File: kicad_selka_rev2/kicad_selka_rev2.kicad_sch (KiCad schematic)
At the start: 104 parts, among them J1 Conn_01x02_Pin, J10 Conn_01x01_Pin, J11 Conn_01x01_Pin, J12 Conn_01x01_Pin, J13 Conn_01x01_Pin, J14 Conn_01x01_Pin, J15 Conn_01x01_Pin, J16 Conn_01x01_Pin, J17 Conn_01x01_Pin, J18 Conn_01x01_Pin, J19 Conn_01x01_Pin, J2 Conn_01x01_Pin, J20 Conn_01x01_Pin, J3 Conn_01x01_Pin, J4 Conn_01x06_Pin, J5 Conn_01x01_Pin, J6 Conn_01x01_Pin, J7 Conn_01x01_Pin, J8 Conn_01x01_Pin, J9 Conn_01x01_Pin, Q1 NPN, U1 ATtiny861A-S

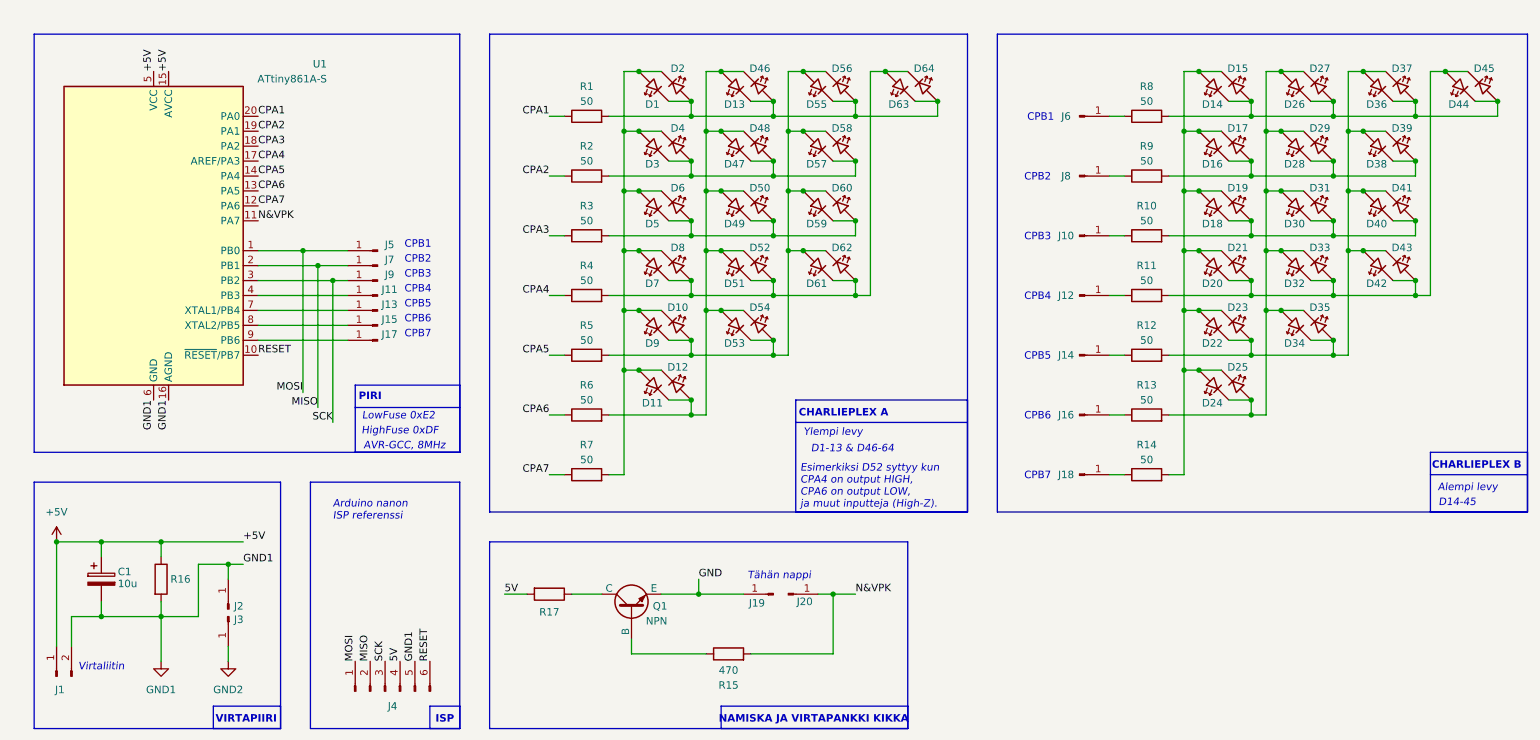
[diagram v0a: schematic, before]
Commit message: hiomista vaille rev
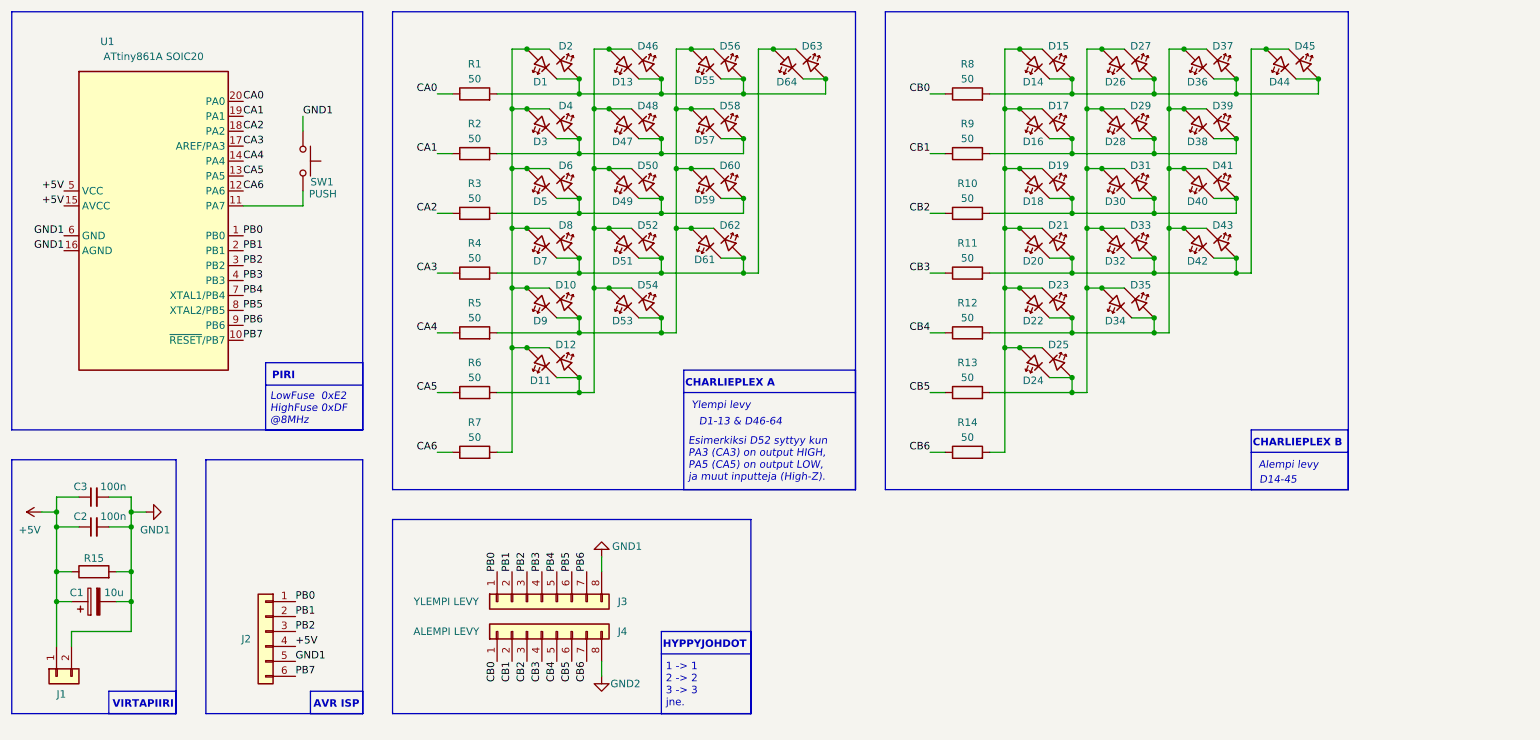
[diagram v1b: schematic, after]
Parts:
- removed J1: Conn_01x02_Pin, Connector_PinHeader_2.00mm:PinHeader_1x02_P2.00mm_Vertical, symbol Connector:Conn_01x02_Pin
- removed J10, J11, J12, J13, J14, J15, J16, J17, J18, J19, J2, J20, J3, J5, J6, J7, J8, J9: Conn_01x01_Pin, Connector_PinHeader_2.00mm:PinHeader_1x01_P2.00mm_Vertical, symbol Connector:Conn_01x01_Pin
- removed J4: Conn_01x06_Pin, Library_zani:PinHeader_1x06_P2.00mm_Horizontal_with_SMD, symbol Connector:Conn_01x06_Pin
- removed Q1: NPN, Package_TO_SOT_SMD:SOT-23_Handsoldering, symbol Simulation_SPICE:NPN
- removed R15: 470, Resistor_SMD:R_1206_3216Metric_Pad1.30x1.75mm_HandSolder, symbol Device:R
- removed R17: X, Resistor_SMD:R_1206_3216Metric_Pad1.30x1.75mm_HandSolder, symbol Device:R
- removed U1: ATtiny861A-S, Package_SO:SOIC-20W_7.5x12.8mm_P1.27mm, symbol MCU_Microchip_ATtiny:ATtiny861A-S
- added C2, C3: 100n, Capacitor_SMD:C_0805_2012Metric_Pad1.18x1.45mm_HandSolder, symbol Device:C_Small
- added J1: Conn_01x02, Connector_PinHeader_2.54mm:PinHeader_1x02_P2.54mm_Vertical, symbol Connector_Generic:Conn_01x02
- added J2: Conn_01x06, footprintteja:PinHeader_1x06_P2.00mm_Horizontal_smd_tht, symbol Connector_Generic:Conn_01x06
- added J3, J4: Conn_01x08, footprintteja:PinHeader_1x08_P2.00mm_Vertical_levee, symbol Connector_Generic:Conn_01x08
- added SW1: PUSH, Connector_PinHeader_2.00mm:PinHeader_1x02_P2.00mm_Vertical, symbol Switch:SW_Push
- added U1: ATtiny861A SOIC20, Package_SO:SOIC-20W_7.5x12.8mm_P1.27mm, symbol ATtiny_861A:ATtiny861A-S
- R15: renamed from R16; footprint Resistor_SMD:R_1206_3216Metric_Pad1.30x1.75mm_HandSolder -> Resistor_SMD:R_1210_3225Metric_Pad1.30x2.65mm_HandSolder
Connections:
- net +5V: now also C2.1, C3.1, J1.1 (Pin_1), J2.4 (Pin_4), U1.15 (AVCC), U1.5 (VCC)
- net GND1: now also C2.2, C3.2, J1.2 (Pin_2), J2.5 (Pin_5), J3.8 (Pin_8), SW1.1, U1.16 (AGND), U1.6 (GND)
- net GND2: now also J4.8 (Pin_8)
- net CB6: now reaches R14.1
- net CB6: now also J4.7 (Pin_7)
- net at D1.1 (K), D13.1 (K), D2.2 (A)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: now also D63.2 (A), D64.1 (K); no longer D63.1 (K), D64.2 (A)
- net CB2: now reaches R10.1
- net CB2: now also J4.3 (Pin_3)
- net at D51.1 (K), D52.2 (A), D61.1 (K)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: now also D63.1 (K), D64.2 (A); no longer D63.2 (A), D64.1 (K)
- net CB3: now reaches R11.1
- net CB3: now also J4.4 (Pin_4)
- net CB1: now reaches R9.1
- net CB1: now also J4.2 (Pin_2)
- net CB0: now reaches R8.1
- net CB0: now also J4.1 (Pin_1)
- net CB4: now reaches R12.1
- net CB4: now also J4.5 (Pin_5)
- net CB5: now reaches R13.1
- net CB5: now also J4.6 (Pin_6)
- net CPA1 renamed CA0
- net CA0: now also U1.20 (PA0)
- net CPA2 renamed CA1
- net CA1: now also U1.19 (PA1)
- net CPA3 renamed CA2
- net CA2: now also U1.18 (PA2)
- net CPA4 renamed CA3
- net CA3: now also U1.17 (AREF/PA3)
- net CPA5 renamed CA4
- net CA4: now also U1.14 (PA4)
- net CPA6 renamed CA5
- net CA5: now also U1.13 (PA5)
- net CPA7 renamed CA6
- net CA6: now also U1.12 (PA6)
- new net: SW1.2, U1.11 (PA7)
- new net PB0: J2.1 (Pin_1), J3.1 (Pin_1), U1.1 (PB0)
- new net PB1: J2.2 (Pin_2), J3.2 (Pin_2), U1.2 (PB1)
- new net PB2: J2.3 (Pin_3), J3.3 (Pin_3), U1.3 (PB2)
- new net PB3: J3.4 (Pin_4), U1.4 (PB3)
- new net PB4: J3.5 (Pin_5), U1.7 (XTAL1/PB4)
- new net PB5: J3.6 (Pin_6), U1.8 (XTAL2/PB5)
- new net PB6: J3.7 (Pin_7), U1.9 (PB6)
- new net PB7: J2.6 (Pin_6), U1.10 (~{RESET}/PB7)
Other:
- note added: "1 -> 1 2 -> 2 3 -> 3 jne."
- note added: "AVR ISP"
- note added: "Esimerkiksi D52 syttyy kun PA3 (CA3) on output HIGH, PA5 (CA5) on output LOW, ja muut inputteja (High-Z)."
- note added: "HYPPYJOHDOT"
- note added: "LowFuse 0xE2 HighFuse 0xDF @8MHz"
- note removed: "AVR-GCC, 8MHz"
- note removed: "Arduino nanon ISP referenssi"
- note removed: "CPB1"
- note removed: "CPB2"
- note removed: "CPB3"
- note removed: "CPB4"
- note removed: "CPB5"
- note removed: "CPB6"
- note removed: "CPB7"
- note removed: "Esimerkiksi D52 syttyy kun CPA4 on output HIGH, CPA6 on output LOW, ja muut inputteja (High-Z)."
- note removed: "HighFuse 0xDF"
- note removed: "ISP"
- note removed: "LowFuse 0xE2"
- note removed: "NAMISKA JA VIRTAPANKKI KIKKA"
- note removed: "Tähän nappi"
- note removed: "Virtaliitin"
- moved on the sheet: C1, D1, D10, D11, D12, D13, D14, D15, D16, D17, D18, D19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
